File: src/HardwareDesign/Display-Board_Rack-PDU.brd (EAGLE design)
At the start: 81.3 x 35.6 mm, 46 parts

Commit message: first order send to JLCPCB
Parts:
- BUT+1, BUT-1, BUT_PWR1, BUT_SET1: value ADTSMW64 -> TC-6601-5.0-160
- ETH: value (none) -> XL-2012UBC
- FAULT: value (none) -> XL-2012SURC
- IC1: value (none) -> MCP23S18-E/MJ
- R26, R27: value 742C083103JP -> 4D03WGJ0102T5E 1K
- R28, R29, R30: value 10K -> 1K
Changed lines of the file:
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@@
 <drawing>
 <settings>
-<setting alwaysvectorfont="yes"/>
+<setting alwaysvectorfont="no"/>
 <setting verticaltext="up"/>
 </settings>
@@
 <element name="CON3" library="ds_con" package="2X7-SIDE" package3d_urn="urn:adsk.eagle:package:46762478/3" value="" x="50.8" y="0" smashed="yes" rot="R270"/>
 <element name="CON4" library="ds_con" package="2X7-SIDE" package3d_urn="urn:adsk.eagle:package:46762478/3" value="" x="71.12" y="0" smashed="yes" rot="R270"/>
-<element name="BUT+1" library="Wurth_Switch_WS-TASV" library_urn="urn:adsk.eagle:library:18304196" package="430182043816" package3d_urn="urn:adsk.eagle:package:18304300/2" value="ADTSMW64" x="43.18" y="27.34" smashed="yes" rot="MR0">
+<element name="BUT+1" library="Wurth_Switch_WS-TASV" library_urn="urn:adsk.eagle:library:18304196" package="430182043816" package3d_urn="urn:adsk.eagle:package:18304300/2" value="TC-6601-5.0-160" x="43.18" y="27.34" smashed="yes" rot="MR0">
 <attribute name="DATASHEET-URL" value="https://www.we-online.com/redexpert/spec/430182043816?ae" x="43.18" y="27.34" size="1.778" layer="28" rot="MR0" display="off"/>
 <attribute name="HEIGHT" value="4.3mm" x="43.18" y="27.34" size="1.778" layer="28" rot="MR0" display="off"/>
@@
 <attribute name="VALUE" x="40.459" y="26.999" size="1.016" layer="27" rot="R270"/>
 </element>
-<element name="BUT-1" library="Wurth_Switch_WS-TASV" library_urn="urn:adsk.eagle:library:18304196" package="430182043816" package3d_urn="urn:adsk.eagle:package:18304300/2" value="ADTSMW64" x="43.18" y="17.78" smashed="yes" rot="MR180">
+<element name="BUT-1" library="Wurth_Switch_WS-TASV" library_urn="urn:adsk.eagle:library:18304196" package="430182043816" package3d_urn="urn:adsk.eagle:package:18304300/2" value="TC-6601-5.0-160" x="43.18" y="17.78" smashed="yes" rot="MR180">
 <attribute name="DATASHEET-URL" value="https://www.we-online.com/redexpert/spec/430182043816?ae" x="33.02" y="5.08" size="1.778" layer="28" rot="MR180" display="off"/>
 <attribute name="HEIGHT" value="4.3mm" x="33.02" y="5.08" size="1.778" layer="28" rot="MR180" display="off"/>
@@
 <attribute name="VALUE" x="44.069" y="15.621" size="1.016" layer="27" rot="R90"/>
 </element>
-<element name="BUT_SET1" library="Wurth_Switch_WS-TASV" library_urn="urn:adsk.eagle:library:18304196" package="430182043816" package3d_urn="urn:adsk.eagle:package:18304300/2" value="ADTSMW64" x="30.48" y="22.86" smashed="yes" rot="MR180">
+<element name="BUT_SET1" library="Wurth_Switch_WS-TASV" library_urn="urn:adsk.eagle:library:18304196" package="430182043816" package3d_urn="urn:adsk.eagle:package:18304300/2" value="TC-6601-5.0-160" x="30.48" y="22.86" smashed="yes" rot="MR180">
 <attribute name="DATASHEET-URL" value="https://www.we-online.com/redexpert/spec/430182043816?ae" x="19.05" y="10.16" size="1.778" layer="28" rot="MR180" display="off"/>
 <attribute name="HEIGHT" value="4.3mm" x="19.05" y="10.16" size="1.778" layer="28" rot="MR180" display="off"/>
@@
 <attribute name="VALUE" x="34.671" y="18.161" size="1.016" layer="27" rot="R90"/>
 </element>
-<element name="BUT_PWR1" library="Wurth_Switch_WS-TASV" library_urn="urn:adsk.eagle:library:18304196" package="430182043816" package3d_urn="urn:adsk.eagle:package:18304300/2" value="ADTSMW64" x="8.89" y="7.62" smashed="yes" rot="MR0">
+<element name="BUT_PWR1" library="Wurth_Switch_WS-TASV" library_urn="urn:adsk.eagle:library:18304196" package="430182043816" package3d_urn="urn:adsk.eagle:package:18304300/2" value="TC-6601-5.0-160" x="8.89" y="7.62" smashed="yes" rot="MR0">
 <attribute name="DATASHEET-URL" value="https://www.we-online.com/redexpert/spec/430182043816?ae" x="30.48" y="21.59" size="1.778" layer="28" rot="MR0" display="off"/>
 <attribute name="HEIGHT" value="4.3mm" x="30.48" y="21.59" size="1.778" layer="28" rot="MR0" display="off"/>
@@
 <attribute name="VALUE" x="12.092075" y="27.94" size="1.016" layer="27" rot="R135"/>
 </element>
-<element name="IC1" library="ds_ic_peripherals" package="QFN50P400X400X100-25T265" package3d_urn="urn:adsk.eagle:package:46683902/2" value="" x="14.04439375" y="30.449184375" smashed="yes" rot="R315">
+<element name="IC1" library="ds_ic_peripherals" package="QFN50P400X400X100-25T265" package3d_urn="urn:adsk.eagle:package:46683902/2" value="MCP23S18-E/MJ" x="14.04439375" y="30.449184375" smashed="yes" rot="R315">
 <attribute name="NAME" x="17.55988125" y="28.483228125" size="1.27" layer="25" rot="R45" align="bottom-center"/>
 <attribute name="VALUE" x="6.541353125" y="33.72245" size="1.27" layer="27" rot="R315" align="top-center"/>
@@
 <attribute name="VALUE" x="58.03" y="12.98" size="0.8128" layer="28" rot="MR180"/>
 </element>
-<element name="R26" library="Resistor Array" library_urn="urn:adsk.eagle:library:16491332" package="742C083103JP" package3d_urn="urn:adsk.eagle:package:16445849/4" value="742C083103JP" x="21.844" y="28.448" smashed="yes" rot="R270">
+<element name="R26" library="Resistor Array" library_urn="urn:adsk.eagle:library:16491332" package="742C083103JP" package3d_urn="urn:adsk.eagle:package:16445849/4" value="4D03WGJ0102T5E 1K" x="21.844" y="28.448" smashed="yes" rot="R270">
 <attribute name="CREATED_BY" value="PCBLayout.com" x="21.844" y="28.448" size="1.778" layer="27" rot="R270" display="off"/>
 <attribute name="DIGIKEY_PN" value="742C083103JPTR-ND" x="21.844" y="28.448" size="1.778" layer="27" rot="R270" display="off"/>
@@
 <attribute name="VALUE" x="19.454390625" y="30.222390625" size="0.66234375" layer="27" rot="R270"/>
 </element>
-<element name="R27" library="Resistor Array" library_urn="urn:adsk.eagle:library:16491332" package="742C083103JP" package3d_urn="urn:adsk.eagle:package:16445849/4" value="742C083103JP" x="21.844" y="32.512" smashed="yes" rot="R270">
+<element name="R27" library="Resistor Array" library_urn="urn:adsk.eagle:library:16491332" package="742C083103JP" package3d_urn="urn:adsk.eagle:package:16445849/4" value="4D03WGJ0102T5E 1K" x="21.844" y="32.512" smashed="yes" rot="R270">
 <attribute name="CREATED_BY" value="PCBLayout.com" x="21.844" y="32.512" size="1.778" layer="27" rot="R270" display="off"/>
 <attribute name="DIGIKEY_PN" value="742C083103JPTR-ND" x="21.844" y="32.512" size="1.778" layer="27" rot="R270" display="off"/>
@@
 <attribute name="VALUE" x="19.454390625" y="34.286390625" size="0.66234375" layer="27" rot="R270"/>
 </element>
-<element name="R28" library="ds_passive" package="0402" package3d_urn="urn:adsk.eagle:package:46683744/2" value="10K" x="4.26" y="22.8" smashed="yes" rot="R270">
+<element name="R28" library="ds_passive" package="0402" package3d_urn="urn:adsk.eagle:package:46683744/2" value="1K" x="4.26" y="22.8" smashed="yes" rot="R270">
 <attribute name="NAME" x="4.895" y="23.435" size="1.016" layer="25" rot="R270"/>
 <attribute name="VALUE" x="2.355" y="23.435" size="1.016" layer="27" rot="R270"/>
 </element>
-<element name="R29" library="ds_passive" package="0402" package3d_urn="urn:adsk.eagle:package:46683744/2" value="10K" x="9.98" y="33.55" smashed="yes" rot="R180">
+<element name="R29" library="ds_passive" package="0402" package3d_urn="urn:adsk.eagle:package:46683744/2" value="1K" x="9.98" y="33.55" smashed="yes" rot="R180">
 <attribute name="NAME" x="10.615" y="32.915" size="1.016" layer="25" rot="R180"/>
 <attribute name="VALUE" x="10.615" y="35.455" size="1.016" layer="27" rot="R180"/>
 </element>
-<element name="R30" library="ds_passive" package="0402" package3d_urn="urn:adsk.eagle:package:46683744/2" value="10K" x="4.24" y="16.26" smashed="yes" rot="R270">
+<element name="R30" library="ds_passive" package="0402" package3d_urn="urn:adsk.eagle:package:46683744/2" value="1K" x="4.24" y="16.26" smashed="yes" rot="R270">
 <attribute name="NAME" x="4.875" y="16.895" size="1.016" layer="25" rot="R270"/>
 <attribute name="VALUE" x="2.335" y="16.895" size="1.016" layer="27" rot="R270"/>
 </element>
-<element name="FAULT" library="led" library_urn="urn:adsk.eagle:library:259" package="CHIP-LED0805" package3d_urn="urn:adsk.eagle:package:15818/2" value="" x="18.04" y="33.54" smashed="yes" rot="MR90">
+<element name="FAULT" library="led" library_urn="urn:adsk.eagle:library:259" package="CHIP-LED0805" package3d_urn="urn:adsk.eagle:package:15818/2" value="XL-2012SURC" x="18.04" y="33.54" smashed="yes" rot="MR90">
 <attribute name="NAME" x="20.83" y="31.17" size="1.27" layer="26" rot="MR0"/>
 <attribute name="VALUE" x="16.77" y="36.08" size="1.27" layer="28" rot="MR180"/>
 </element>
-<element name="ETH" library="led" library_urn="urn:adsk.eagle:library:259" package="CHIP-LED0805" package3d_urn="urn:adsk.eagle:package:15818/2" value="" x="8.52" y="21.49" smashed="yes" rot="MR90">
+<element name="ETH" library="led" library_urn="urn:adsk.eagle:library:259" package="CHIP-LED0805" package3d_urn="urn:adsk.eagle:package:15818/2" value="XL-2012UBC" x="8.52" y="21.49" smashed="yes" rot="MR90">
 <attribute name="NAME" x="10.65" y="22.22" size="1.27" layer="26" rot="MR180"/>
 <attribute name="VALUE" x="7.25" y="24.03" size="1.27" layer="28" rot="MR180"/>

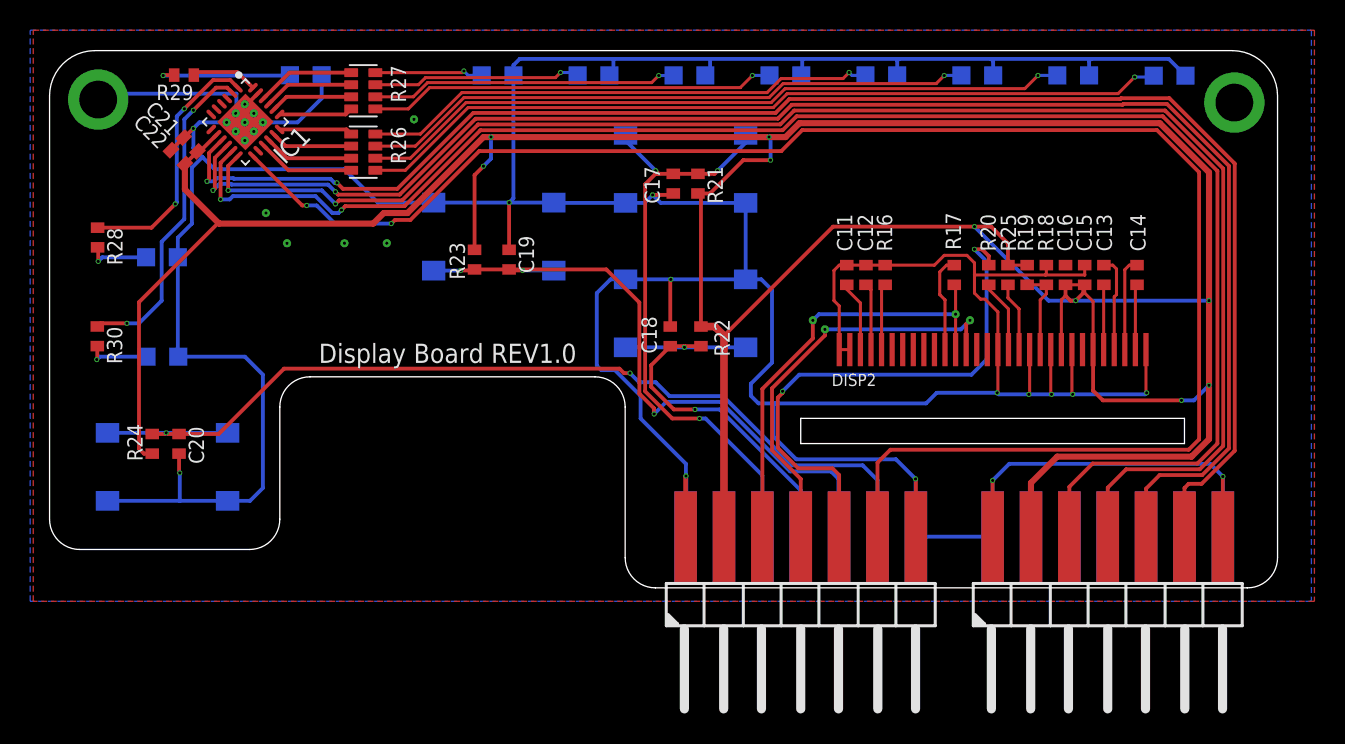
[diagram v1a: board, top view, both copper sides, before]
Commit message: generate Gerber files
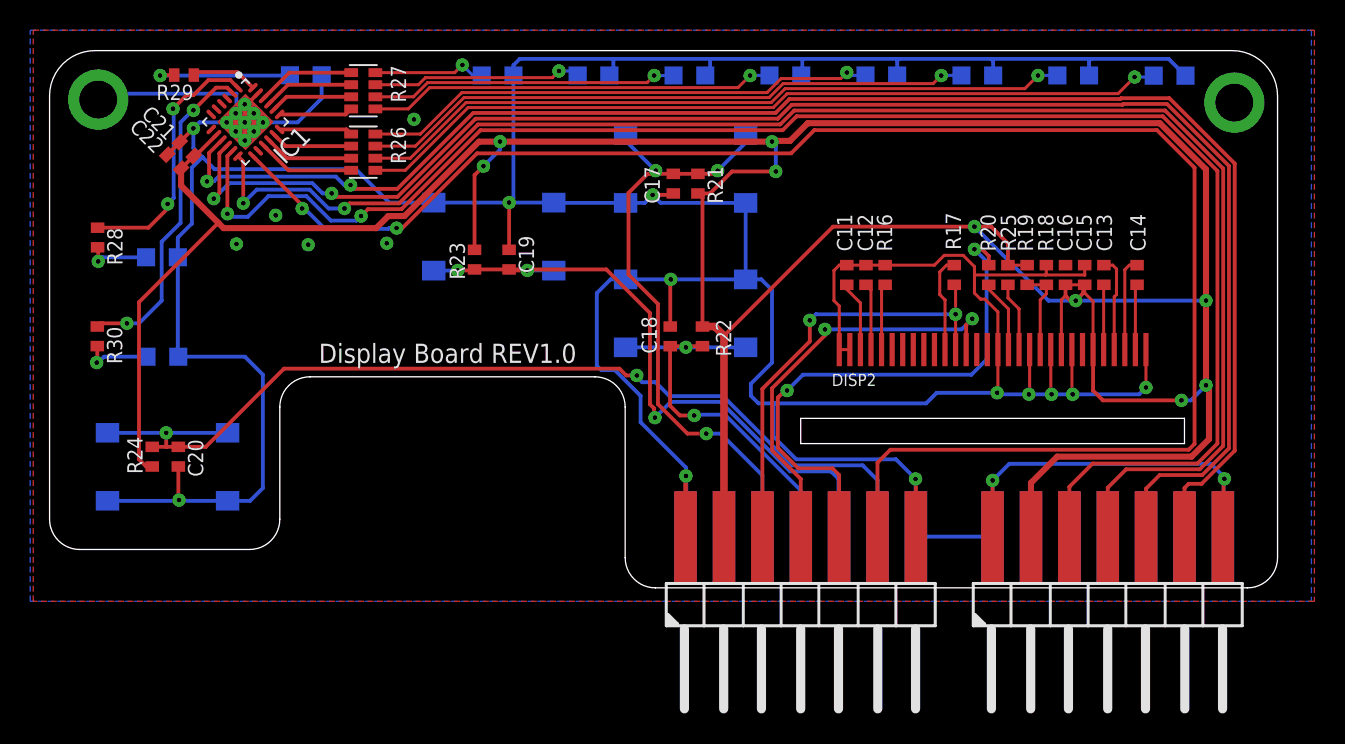
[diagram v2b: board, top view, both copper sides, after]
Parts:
- moved C20 0.85 mm to (9.60, 8.29)
- moved R24 0.85 mm to (7.87, 8.29)
- moved C21 0.39 mm to (10.2, 28.7)
- moved C22 0.39 mm to (9.33, 27.8)
- moved R22 0.10 mm to (44.3, 16.3)
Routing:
- net SPI_MOSI: track 106.6 -> 107.8 mm
- net KEY_3: track 64.6 -> 65.9 mm
- net +3V3: track 234.7 -> 235.9 mm
- net KEY_0: track 39.6 -> 40.8 mm
- net KEY_1: track 29.1 -> 28.2 mm
- net SPI_SCK: track 103.7 -> 104.6 mm
- net GND: track 363.5 -> 362.6 mm
